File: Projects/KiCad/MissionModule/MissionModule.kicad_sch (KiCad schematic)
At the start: 23 parts, among them J1 Conn_01x04_Pin, J2 Conn_01x04_Pin, J3 Micro_SD_Card_Det_Hirose_DM3AT, U1 ABX00012, U2 MCP2562-E-P, U3 LT1584-3.3, U4 TLP222A, U5 MCP2515-I/P, Y1 8MHz

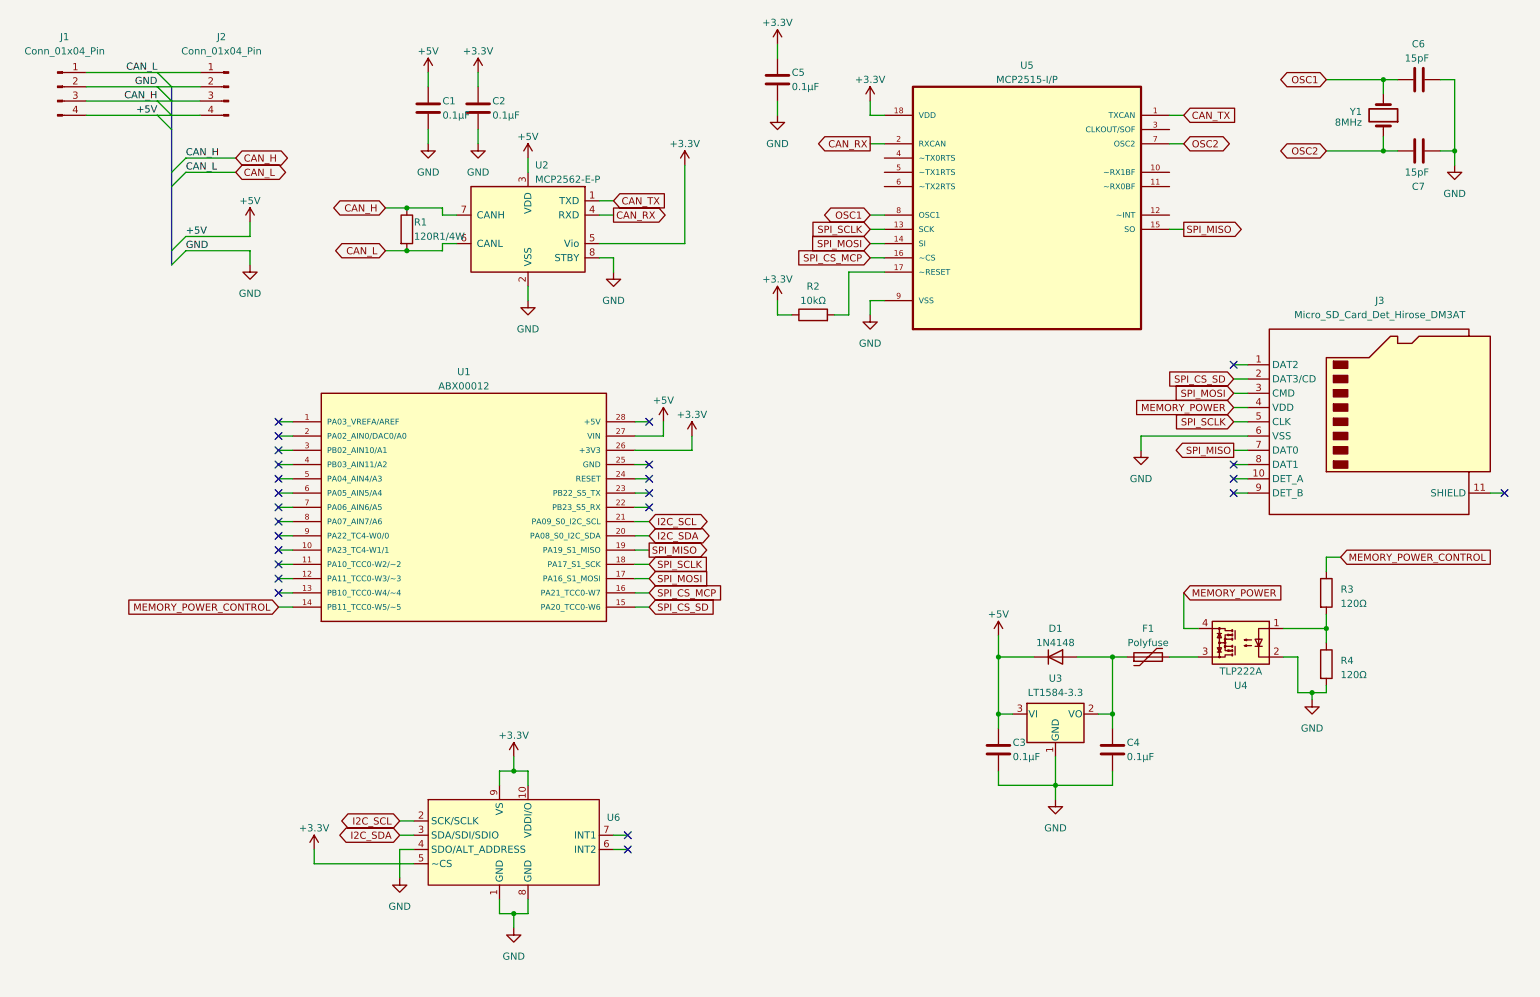
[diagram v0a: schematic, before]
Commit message: 全モジュールのkicadを一通り作った
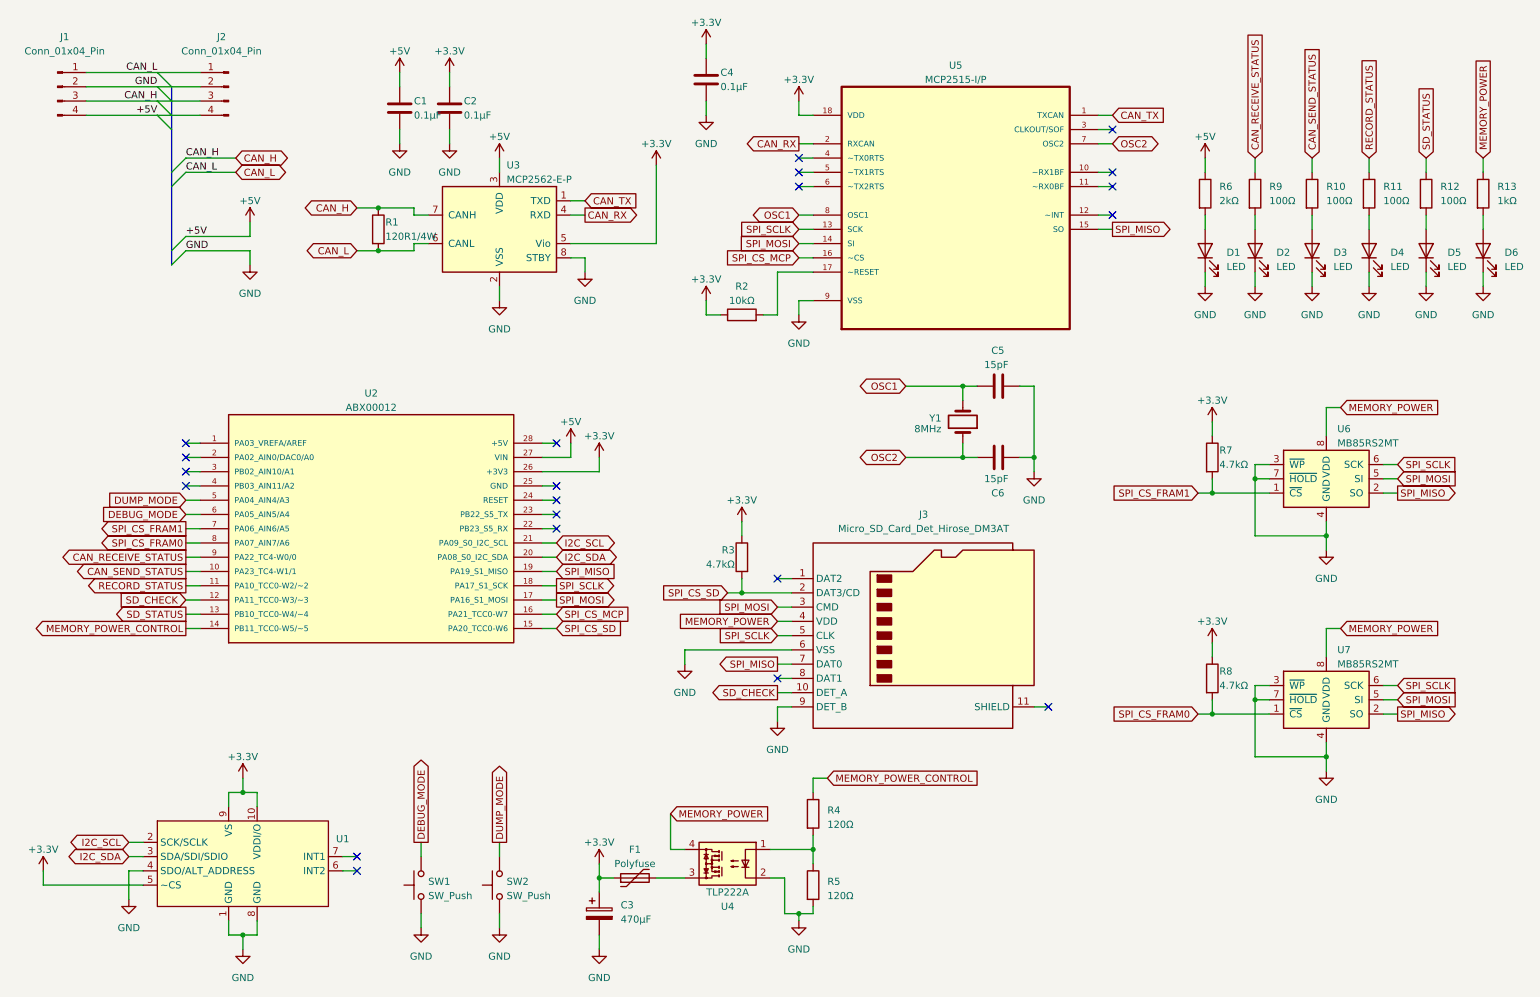
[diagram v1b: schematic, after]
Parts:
- removed C3, C4: 0.1μF, Capacitor_SMD:C_0805_2012Metric_Pad1.18x1.45mm_HandSolder, symbol Device:C
- removed D1: 1N4148, Diode_THT:D_DO-35_SOD27_P7.62mm_Horizontal, symbol Diode:1N4148
- removed U3: LT1584-3.3, Package_TO_SOT_THT:TO-220-3_Vertical, symbol Regulator_Linear:LT1584-3.3
- added C3: 470μF, Capacitor_THT:CP_Radial_D10.0mm_P3.50mm, symbol Device:C_Polarized
- added D1, D2, D3, D4, D5, D6: LED, LED_SMD:LED_1206_3216Metric_Pad1.42x1.75mm_HandSolder, symbol Device:LED
- added R10, R11, R12, R9: 100Ω, Resistor_SMD:R_0805_2012Metric_Pad1.20x1.40mm_HandSolder, symbol Device:R
- added R13: 1kΩ, Resistor_SMD:R_0805_2012Metric_Pad1.20x1.40mm_HandSolder, symbol Device:R
- added R3, R7, R8: 4.7kΩ, Resistor_SMD:R_0805_2012Metric_Pad1.20x1.40mm_HandSolder, symbol Device:R
- added R6: 2kΩ, Resistor_SMD:R_0805_2012Metric_Pad1.20x1.40mm_HandSolder, symbol Device:R
- added SW1, SW2: SW_Push, Button_Switch_THT:SW_PUSH_6mm, symbol Switch:SW_Push
- added U6, U7: MB85RS2MT, Package_DIP:DIP-8_W7.62mm, symbol Memory_NVRAM:MB85RS2MT
- R2: footprint (none) -> Resistor_SMD:R_0805_2012Metric_Pad1.20x1.40mm_HandSolder
- renumbered C5 to C4, C6 to C5, C7 to C6, R3 to R4, R4 to R5, U6 to U1, U1 to U2, U2 to U3
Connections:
- net +3.3V: now also F1.1, C3.1, R3.1, R7.1, R8.1
- net +5V: now also R6.1
- net GND: now also J3.9 (DET_B), C3.2, D1.1 (K), D2.1 (K), D3.1 (K), D4.1 (K), D5.1 (K), D6.1 (K), SW1.1, SW2.1, U6.3 (~{WP}), U6.4 (GND), U6.7 (~{HOLD}), U7.3 (~{WP}), U7.4 (GND), U7.7 (~{HOLD})
- net MEMORY_POWER: now also R13.1, U6.8 (VDD), U7.8 (VDD)
- net SPI_CS_SD: now also R3.2
- net SPI_MISO: now also U6.2 (SO), U7.2 (SO)
- net SPI_MOSI: now also U6.5 (SI), U7.5 (SI)
- net SPI_SCLK: now also U6.6 (SCK), U7.6 (SCK)
- net CAN_SEND_STATUS: now reaches U2.10 (PA23_TC4-W1/1)
- net CAN_SEND_STATUS: now also R10.1
- net RECORD_STATUS: now reaches U2.11 (PA10_TCC0-W2/~2)
- net RECORD_STATUS: now also R11.1
- net SD_CHECK: now reaches U2.12 (PA11_TCC0-W3/~3)
- net SD_CHECK: now also J3.10 (DET_A)
- net SD_STATUS: now reaches U2.13 (PB10_TCC0-W4/~4)
- net SD_STATUS: now also R12.1
- net DUMP_MODE: now reaches U2.5 (PA04_AIN4/A3)
- net DUMP_MODE: now also SW2.2
- net DEBUG_MODE: now reaches U2.6 (PA05_AIN5/A4)
- net DEBUG_MODE: now also SW1.2
- net SPI_CS_FRAM1: now reaches U2.7 (PA06_AIN6/A5)
- net SPI_CS_FRAM1: now also R7.2, U6.1 (~{CS})
- net SPI_CS_FRAM0: now reaches U2.8 (PA07_AIN7/A6)
- net SPI_CS_FRAM0: now also R8.2, U7.1 (~{CS})
- net CAN_RECEIVE_STATUS: now reaches U2.9 (PA22_TC4-W0/0)
- net CAN_RECEIVE_STATUS: now also R9.1
- new net: D1.2 (A), R6.2
- new net: D5.2 (A), R12.2
- new net: D4.2 (A), R11.2
- new net: D3.2 (A), R10.2
- new net: D6.2 (A), R13.2
- new net: D2.2 (A), R9.2
- no-connect marks 25 -> 21
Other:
- moved on the sheet: C1, C2, C4, C5, C6, F1, J3, R1, R2, R4, R5, U1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
